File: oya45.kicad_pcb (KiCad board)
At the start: 2 copper layers, 190.5 x 95.2 mm, 94 parts, among them U1 ProMicro

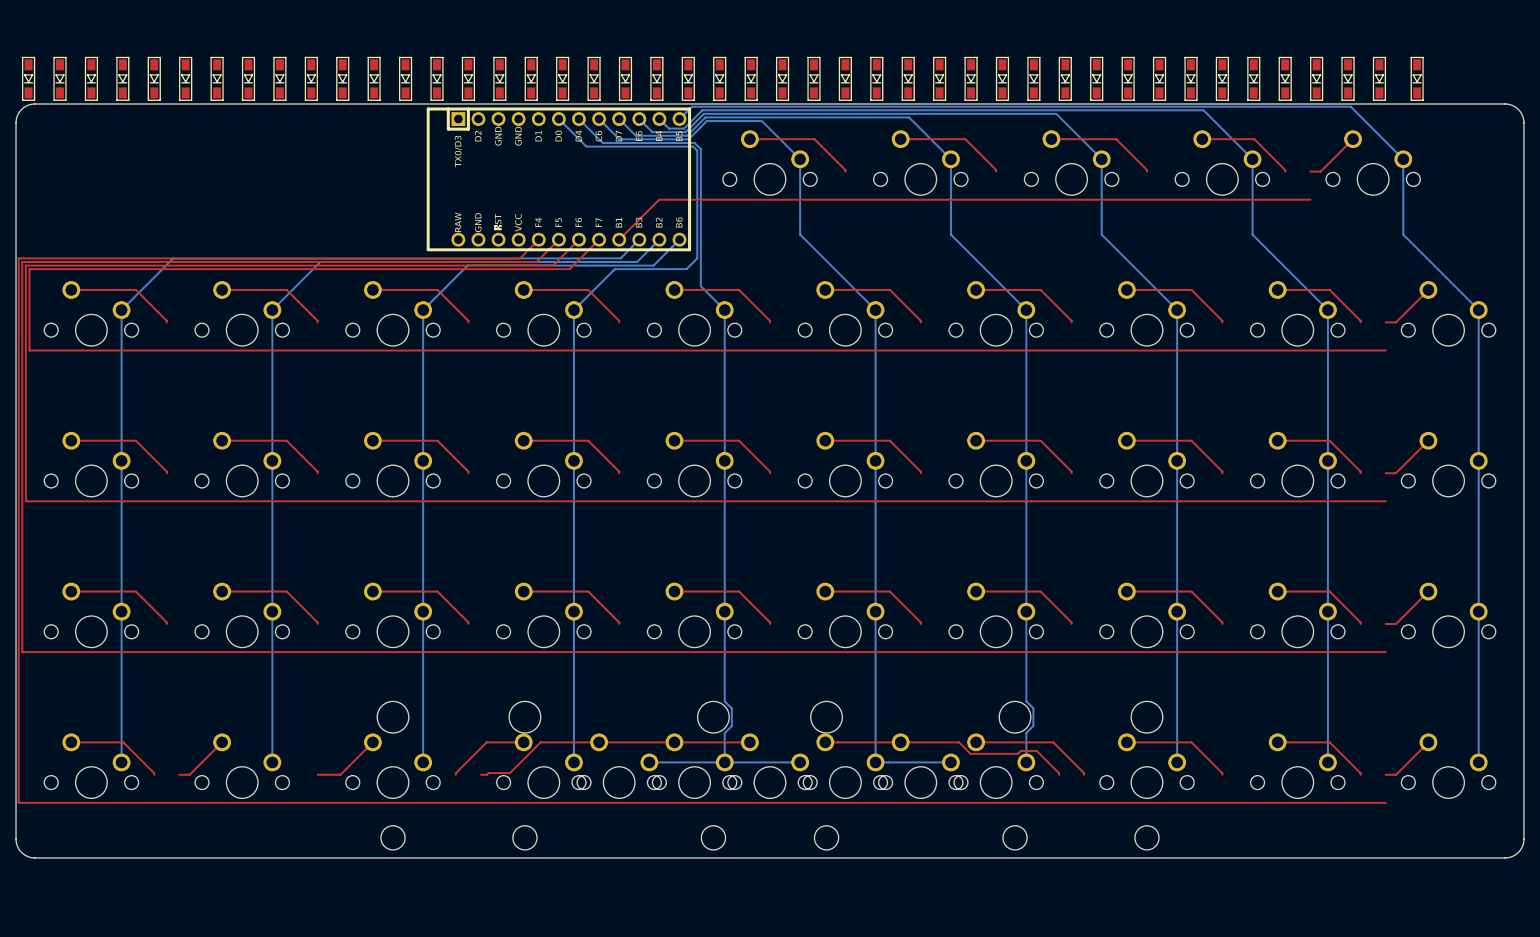
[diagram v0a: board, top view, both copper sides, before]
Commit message: save
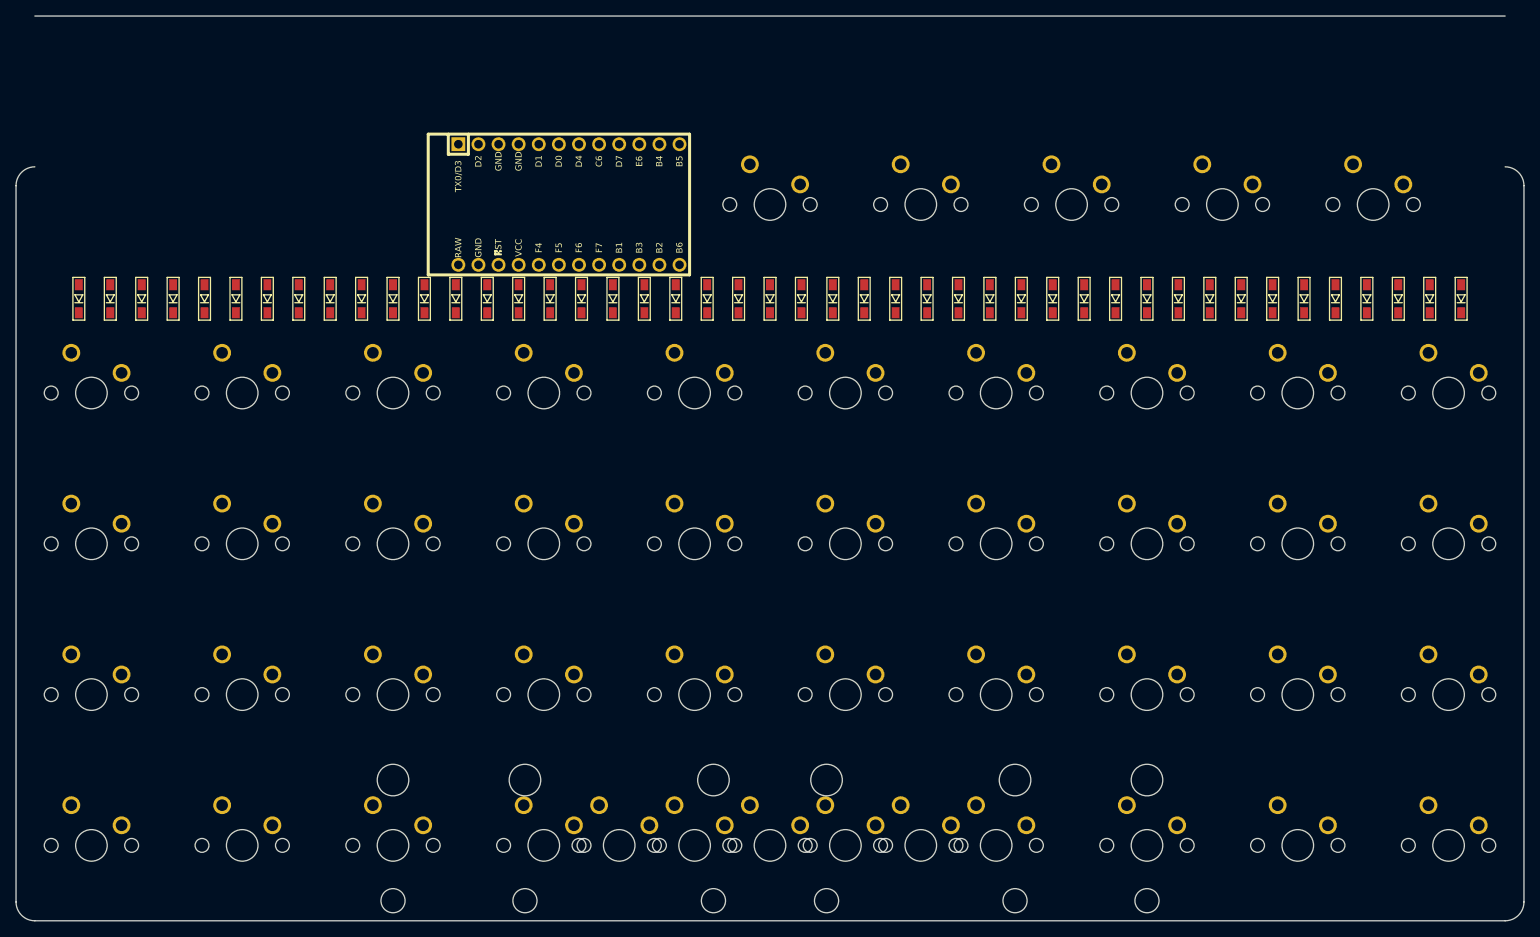
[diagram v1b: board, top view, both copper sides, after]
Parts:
- moved D1 28.5 mm to (55.6, 53.2)
- moved D10 28.5 mm to (91.3, 53.2)
- moved D11 28.5 mm to (95.2, 53.2)
- moved D12 28.5 mm to (99.2, 53.2)
- moved D13 28.5 mm to (103.2, 53.2)
- moved D14 28.5 mm to (107.2, 53.2)
- moved D15 28.5 mm to (111.1, 53.2)
- moved D16 28.5 mm to (115.1, 53.2)
- moved D17 28.5 mm to (119.1, 53.2)
- moved D18 28.5 mm to (123.0, 53.2)
- moved D19 28.5 mm to (127.0, 53.2)
- moved D2 28.5 mm to (59.5, 53.2)
- moved D20 28.5 mm to (131.0, 53.2)
- moved D21 28.5 mm to (134.9, 53.2)
- moved D22 28.5 mm to (138.9, 53.2)
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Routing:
- net row4: track 308.2 -> 0.00 mm
- net row3: track 290.5 -> 0.00 mm
- net row2: track 272.8 -> 0.00 mm
- net row1: track 255.1 -> 0.00 mm
- net col9: track 175.0 -> 0.00 mm
- net col8: track 159.1 -> 0.00 mm
- net col7: track 142.6 -> 0.00 mm
- net col6: track 126.8 -> 0.00 mm
- net col0: track 126.2 -> 0.00 mm
- net col5: track 119.1 -> 0.00 mm
- net col4: track 115.5 -> 0.00 mm
- net col1: track 109.7 -> 0.00 mm
- net col3: track 108.2 -> 0.00 mm
- net col2: track 93.2 -> 0.00 mm
- net row0: track 89.4 -> 0.00 mm
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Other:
- board size 190.5 x 95.2 mm -> 190.5 x 114.3 mm
